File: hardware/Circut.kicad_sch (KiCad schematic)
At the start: 27 parts, among them J1 USB_C_Receptacle_USB2.0_14P, J2 USB_B_Mini, J3 Jack-DC, J4 Conn_01x24_Pin, J5 Conn_01x24_Pin, J6 Conn_01x24_Pin, J7 Conn_01x03_Pin, U1 ESP32-WROOM-32, U2 AMS1117-3.3, U3 AMS1117CD-5.0

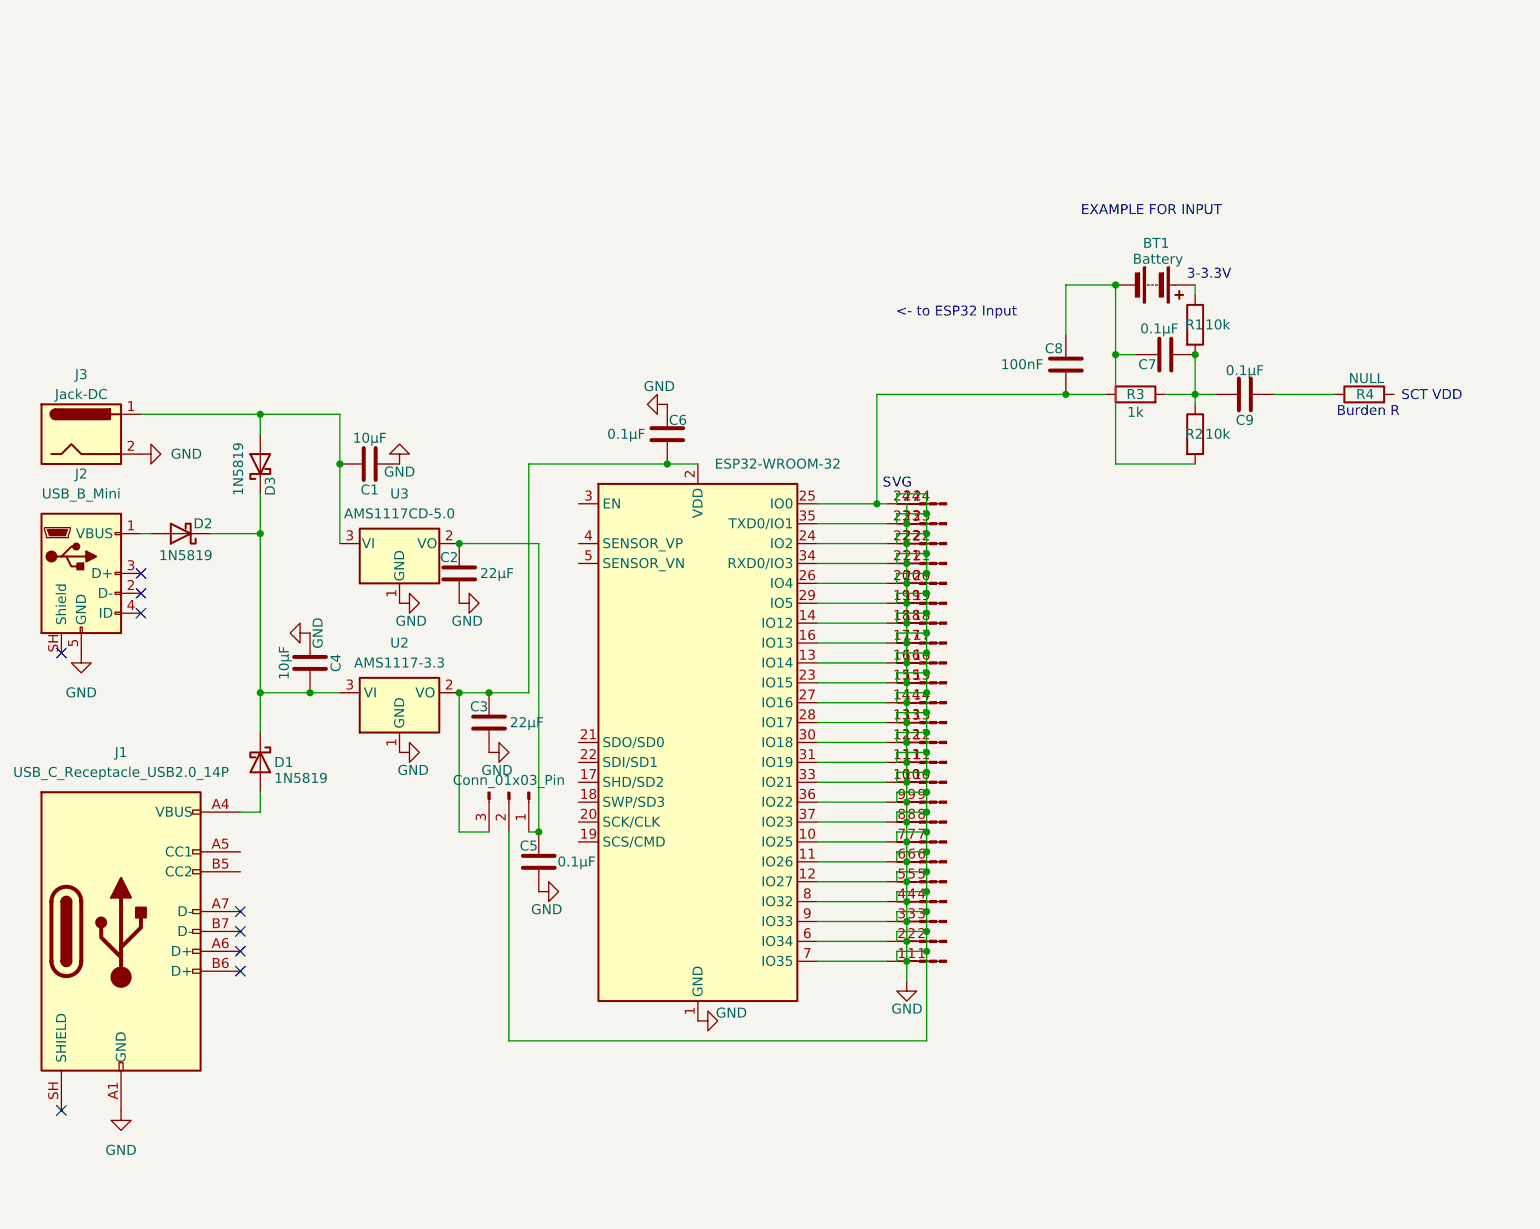
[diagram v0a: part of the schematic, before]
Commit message: Fix: Huge fix for frontend && sensor src && Detail for every folder in project
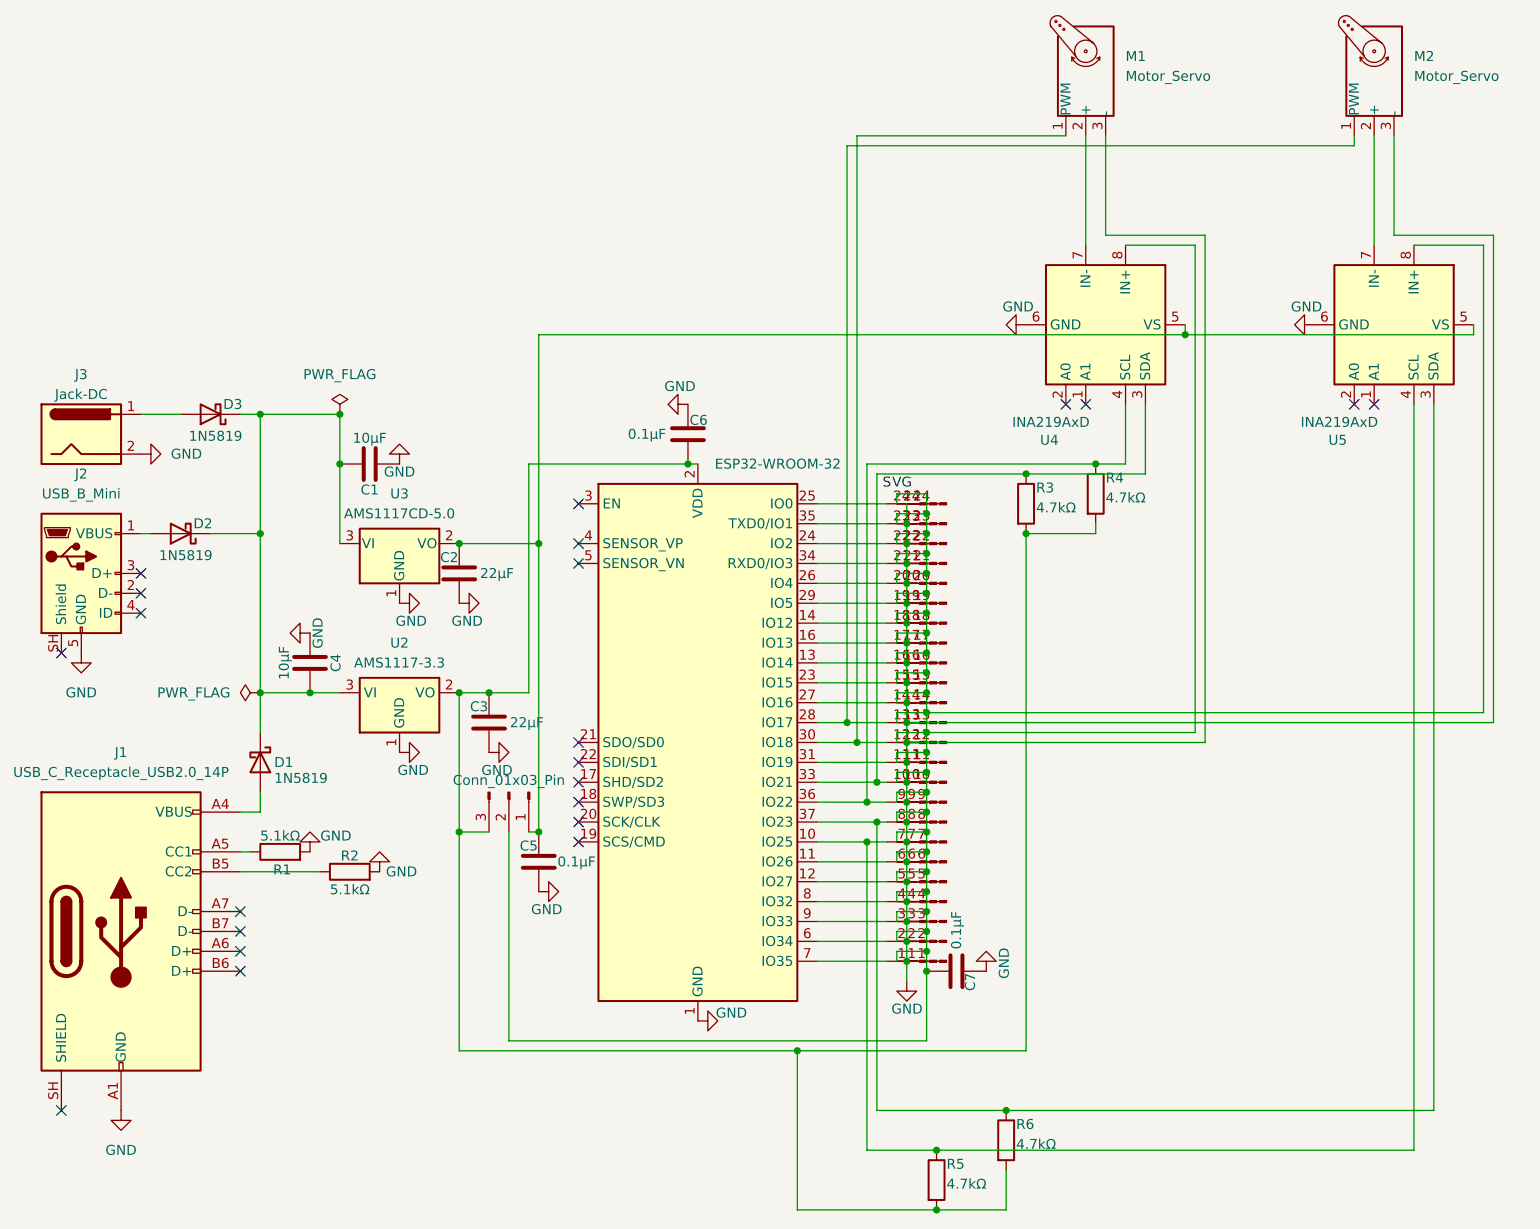
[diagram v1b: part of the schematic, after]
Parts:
- removed BT1: Battery, symbol Device:Battery
- removed C8: 100nF, symbol Device:C
- removed C9: 0.1µF, symbol Device:C
- added M1, M2: Motor_Servo, symbol Motor:Motor_Servo
- added R5, R6: 4.7kΩ, Resistor_SMD:R_0402_1005Metric, symbol Device:R
- added U4, U5: INA219AxD, Package_SO:SOIC-8_3.9x4.9mm_P1.27mm, symbol Sensor_Energy:INA219AxD
- C1, C2, C3, C4, C5, C6, C7: footprint (none) -> Capacitor_SMD:C_0402_1005Metric_Pad0.74x0.62mm_HandSolder
- D1, D2, D3: footprint Diode_THT:D_DO-41_SOD81_P10.16mm_Horizontal -> Diode_SMD:D_0402_1005Metric
- J1: footprint (none) -> Connector_USB:USB_C_Receptacle_GCT_USB4085
- J2: footprint (none) -> Connector_USB:USB_Mini-B_Lumberg_2486_01_Horizontal
- J3: footprint (none) -> Connector_BarrelJack:BarrelJack_CUI_PJ-063AH_Horizontal
- J4: footprint (none) -> Connector_PinHeader_1.00mm:PinHeader_1x24_P1.00mm_Vertical_SMD_Pin1Left
- J5, J6: footprint (none) -> Connector_PinHeader_1.00mm:PinHeader_1x24_P1.00mm_Vertical_SMD_Pin1Right
- J7: footprint (none) -> Connector_PinHeader_1.00mm:PinHeader_1x03_P1.00mm_Horizontal
- R1, R2: value 10k -> 5.1kΩ; footprint (none) -> Resistor_SMD:R_0402_1005Metric
- R3: value 1k -> 4.7kΩ; footprint (none) -> Resistor_SMD:R_0402_1005Metric
- R4: value NULL -> 4.7kΩ; footprint (none) -> Resistor_SMD:R_0402_1005Metric
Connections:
- net GND: now also C7.2, R1.2, R2.2, M1.3 (-), M2.3 (-), U4.6 (GND), U5.6 (GND)
- net at C2.1, C5.1, J7.1 (Pin_1)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: now also U4.5 (VS), U5.5 (VS)
- net at J4.24 (Pin_24), U1.25 (IO0): no longer R3.1
- net at J1.A5 (CC1): now also R1.1
- net at J1.B5 (CC2): now also R2.1
- net at C3.1, C6.1, J7.3 (Pin_3)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: now also R3.2, R4.2, R5.2, R6.2
- net at C1.1, U3.3 (VI): now also C4.1, D1.1 (K), D2.1 (K), D3.1 (K), U2.3 (VI); no longer D3.2 (A), J3.1
- net at R4.1: now also J4.9 (Pin_9), U1.36 (IO22), U4.4 (SCL)
- net at J5.1 (Pin_1), J5.10 (Pin_10), J5.11 (Pin_11)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: now also C7.1, U4.8 (IN+), U5.8 (IN+)
- net at J4.7 (Pin_7), U1.10 (IO25): now also R5.1, U5.4 (SCL)
- net at J4.13 (Pin_13), U1.28 (IO17): now also M2.1 (PWM)
- net at J4.12 (Pin_12), U1.30 (IO18): now also M1.1 (PWM)
- net at J4.10 (Pin_10), U1.33 (IO21): now also R3.1, U4.3 (SDA)
- net at J4.8 (Pin_8), U1.37 (IO23): now also R6.1, U5.3 (SDA)
- new net: M2.2 (+), U5.7 (IN-)
- new net: M1.2 (+), U4.7 (IN-)
- new net: D3.2 (A), J3.1
- no-connect marks 9 -> 22
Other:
- note removed: "3-3.3V"
- note removed: "<- to ESP32 Input"
- note removed: "Burden R"
- note removed: "EXAMPLE FOR INPUT"
- note removed: "SCT VDD"
- moved on the sheet: C6, D3

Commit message: Optimized backend and frontend
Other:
- moved on the sheet: C1, C2, C3, C4, C5, C6, C7, D1, D2, D3, J1, J2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
